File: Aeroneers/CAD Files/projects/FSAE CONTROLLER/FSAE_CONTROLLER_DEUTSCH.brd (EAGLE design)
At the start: 24 parts, among them IC1 MPU-9250, IC2 R-783.3-1.0, U1 DUAL-OPTOISOLATOR_SOIC8

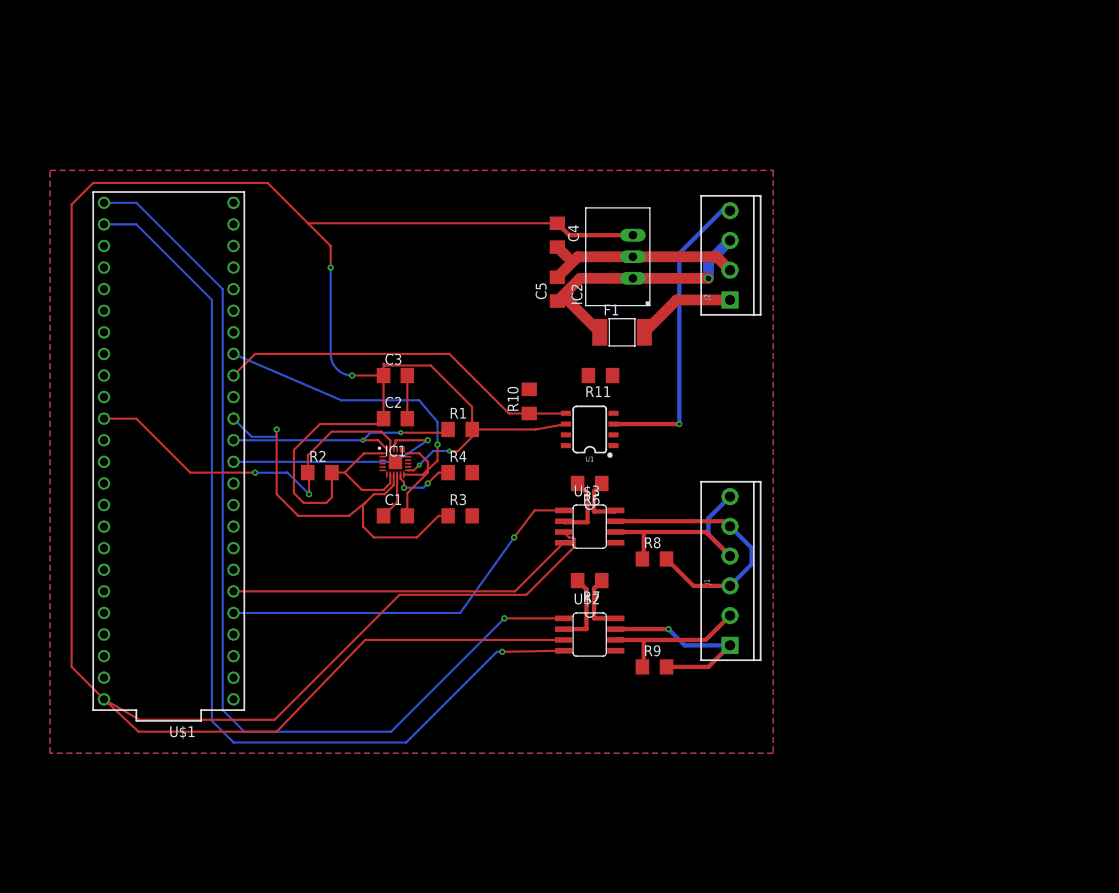
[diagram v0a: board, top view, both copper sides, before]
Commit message: End of semester commit
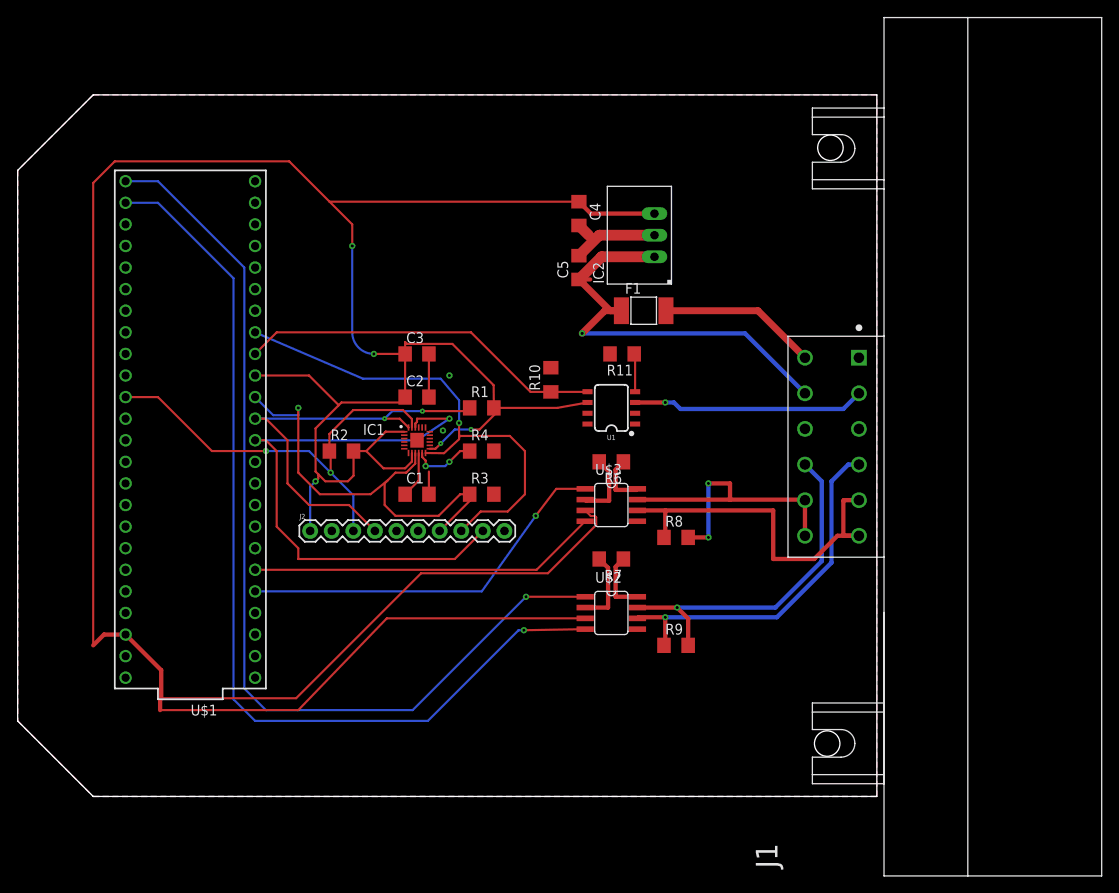
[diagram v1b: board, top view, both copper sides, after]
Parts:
- J1: value (none) -> DTM13-12PA-R008; device SparkFun-Connectors:SCREWTERMINAL-3.5MM-6 -> DTM13-12PA-R008:TE_DTM13-12PA-R008
- J2: device SparkFun-Connectors:SCREWTERMINAL-3.5MM-4 -> SparkFun-Connectors:1X10
- moved J2 56.4 mm to (34.4, 31.2), turned to 0 degrees
- moved J1 26.8 mm to (97.0, 41.1)
- moved IC2 3.59 mm to (74.9, 66.0)
- moved C5 3.59 mm to (66.0, 62.2)
- moved R11 3.59 mm to (71.1, 52.1)
- moved C1 3.59 mm to (47.0, 35.6)
- moved C2 3.59 mm to (47.0, 47.0)
- moved C3 3.59 mm to (47.0, 52.1)
- moved C4 3.59 mm to (66.0, 68.6)
- moved IC1 3.59 mm to (47.0, 41.9)
- moved R1 3.59 mm to (54.6, 45.7)
- moved R10 3.59 mm to (62.7, 49.0)
- moved R2 3.59 mm to (38.1, 40.6)
- moved R3 3.59 mm to (54.6, 35.6)
- moved R4 3.59 mm to (54.6, 40.6)
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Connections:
- removed net 3.3V: U$1.3.3V, U$1.3.3V3
- removed net N$23: F1.2, J2.1
- removed net N$8: IC1.12, U$1.25
- new net N$20: F1.2, J1.12
- new net N$26: IC1.12, J2.8, U$1.25
- new net VIN: U$1.VIN
- net GND: now also J1.1
- net N$1: now also J1.11; no longer J2.3
- net N$14: now also J1.9; no longer J1.1
- net N$15: now also J1.7, J1.8; no longer J1.3, J1.5
- net N$16: now also J1.5; no longer J1.4
- net N$17: now also J1.4; no longer J1.2
- net N$24: now also J1.2; no longer J2.4
- net N$25: now also J2.1, U$1.3.3V, U$1.3.3V3; no longer U$1.VIN
- net N$5: now also J2.3
- net N$6: now also J2.4
- net N$7: now also J2.7
- net N$9: now also J2.9
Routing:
- net N$26: track 0.00 -> 58.4 mm, vias 0 -> 1
- net N$9: track 28.6 -> 68.5 mm
- net N$8: track 35.5 -> 0.00 mm, vias 1 -> 0
- net N$17: track 17.9 -> 42.5 mm, vias 0 -> 1
- net N$6: track 29.0 -> 51.6 mm
- net N$1: track 30.9 -> 53.4 mm
- net GND: track 63.3 -> 43.8 mm, vias 0 -> 2
- net N$20: track 0.00 -> 18.6 mm
- net N$14: track 22.7 -> 41.1 mm
- net N$25: track 363.1 -> 380.7 mm, vias 4 -> 5
- net N$16: track 27.0 -> 44.1 mm
- net N$23: track 11.7 -> 0.00 mm
- net N$24: track 35.9 -> 27.4 mm
- net N$5: track 44.7 -> 52.7 mm
- net N$7: track 46.5 -> 52.3 mm
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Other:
- board outline added: 101.1 x 82.5 mm
